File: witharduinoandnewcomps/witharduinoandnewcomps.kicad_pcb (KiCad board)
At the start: 2 copper layers, 60 x 90 mm, 20 parts, among them J1 FH34SRJ-24S-0.5SH_99_, Q2 ZXM61N03F, Q3 ZXM61N03F, SW1 Button-THT - 2-1825910-7

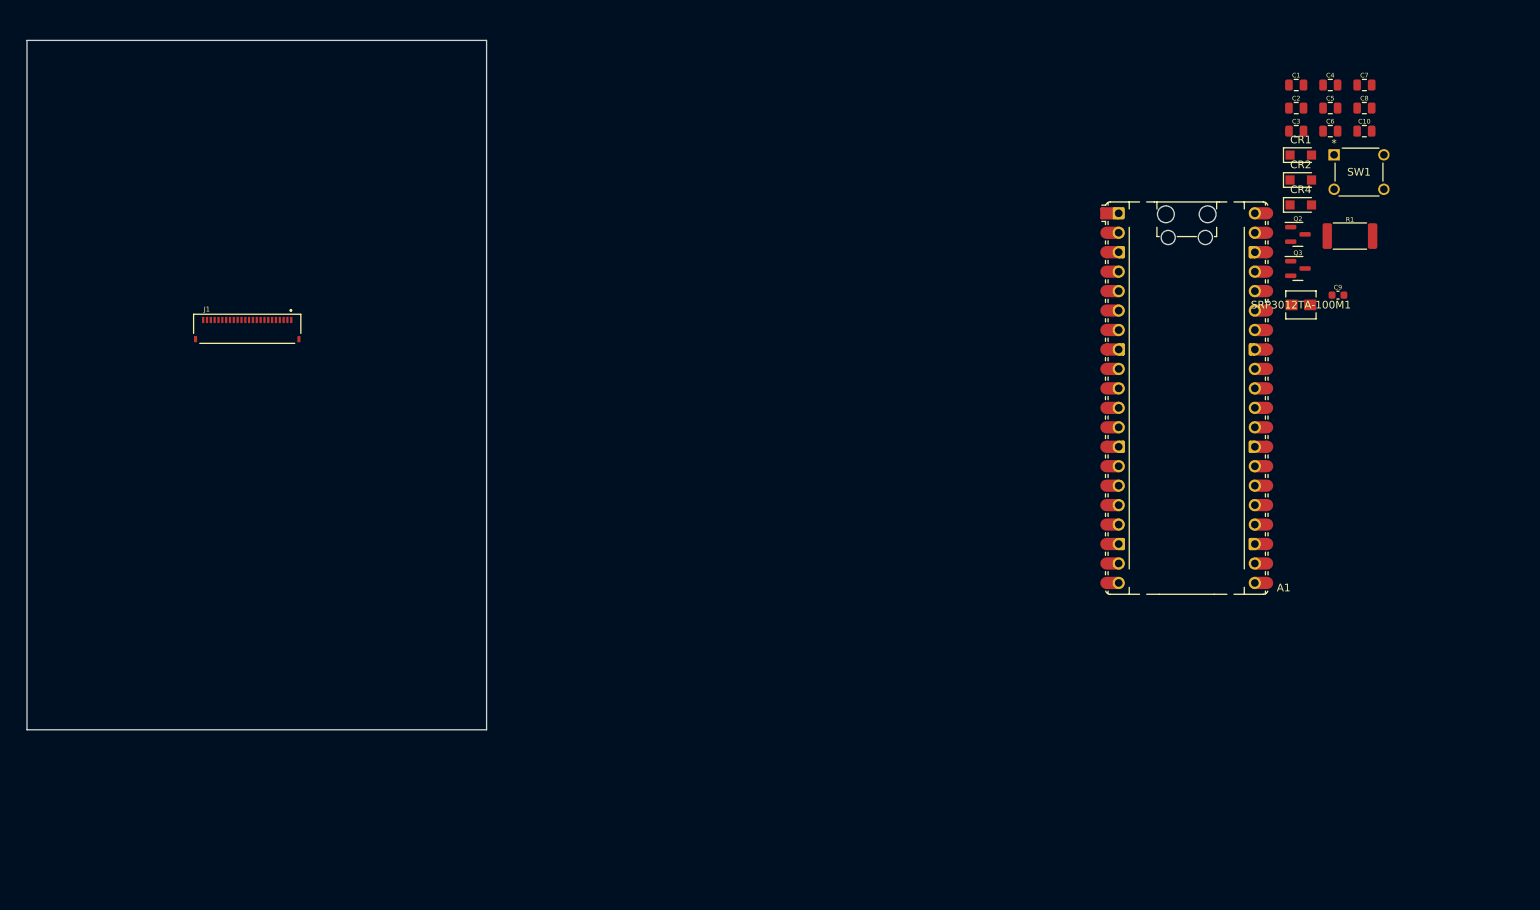
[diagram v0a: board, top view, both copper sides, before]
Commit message: Nov22
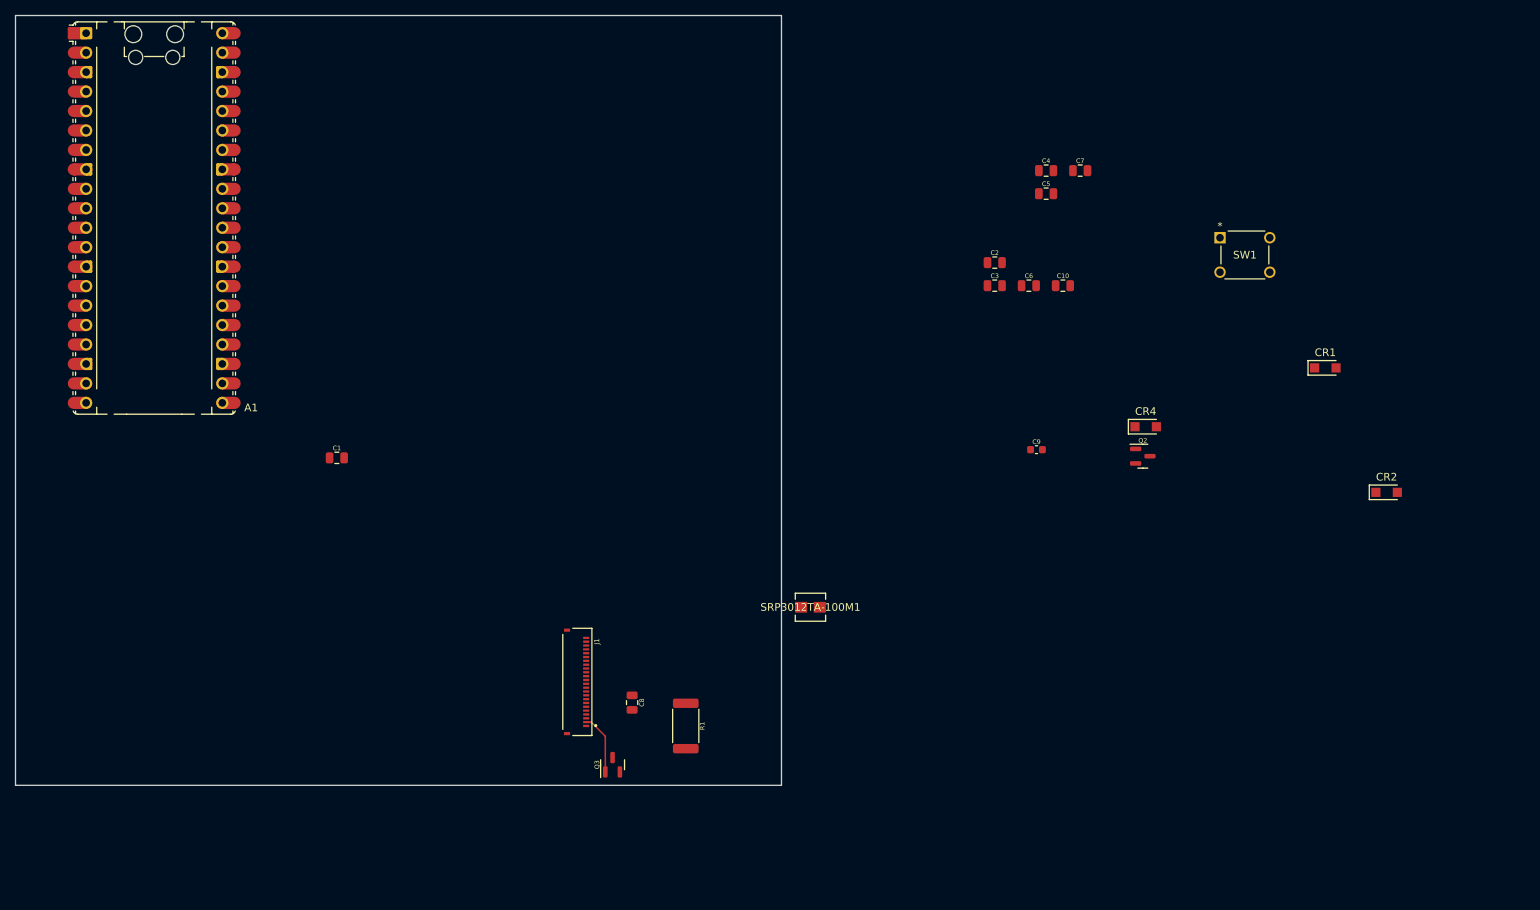
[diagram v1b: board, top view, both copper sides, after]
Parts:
- moved A1 136.8 mm to (44.6, 53.2)
- moved C1 134.4 mm to (68.5, 84.5)
- moved C8 123.1 mm to (107.0, 116.5), turned to -90 degrees
- moved Q3 110.5 mm to (104.5, 124.6), turned to 90 degrees
- moved R1 107.7 mm to (114.0, 119.5), turned to -90 degrees
- moved SRP3012TA-100M1 75.2 mm to (130.3, 104.0)
- moved J1 63.1 mm to (99.8, 113.8), turned to -90 degrees
- moved C6 44.2 mm to (158.8, 62.0)
- moved C9 44.2 mm to (159.8, 83.4)
- moved C10 44.2 mm to (163.2, 62.0)
- moved C2 44.2 mm to (154.3, 59.0)
- moved C3 44.2 mm to (154.3, 62.0)
- moved CR2 42.3 mm to (205.5, 89.0)
- moved C4 38.7 mm to (161.1, 47.0)
- moved C5 38.7 mm to (161.1, 50.0)
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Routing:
- net Net-(Q3-G): track 0.00 -> 7.92 mm
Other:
- board size 60 x 90 mm -> 100 x 100.5 mm

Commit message: laid out pcb
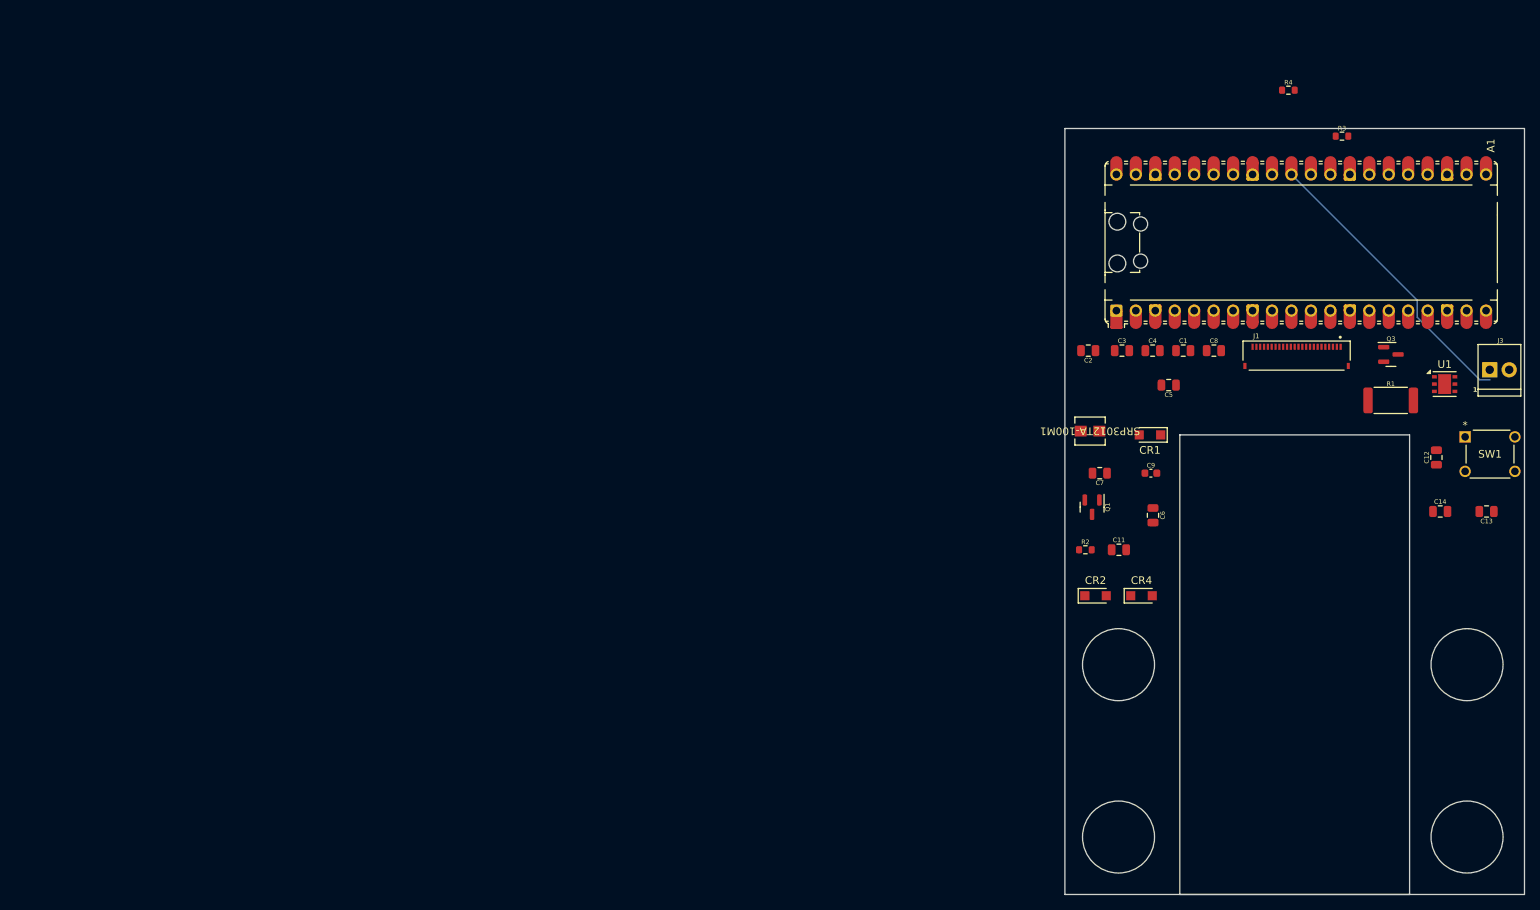
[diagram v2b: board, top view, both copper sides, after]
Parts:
- removed C10: 4u7, rsx_capacitors:C_0805_2012Metric
- removed Q2: ZXM61N03F, rsx_packages_TO_SOT:SOT-23
- added C11: 10u, rsx_capacitors:C_0805_2012Metric, F.Cu at (170.6, 96.5)
- added C12: 1u, rsx_capacitors:C_0805_2012Metric, F.Cu at (212.0, 84.5)
- added C13: 1u, rsx_capacitors:C_0805_2012Metric, F.Cu at (218.6, 91.5)
- added C14: 4u7, rsx_capacitors:C_0805_2012Metric, F.Cu at (212.5, 91.5)
- added J3: Screw_Terminal_2x2.54, rsx_headers_screw:Wurth_691210910002, F.Cu at (219.7, 73.0)
- added Q1: ZXM61N03F, rsx_packages_TO_SOT:SOT-23, F.Cu at (167.1, 90.9)
- added R2: 10k, rsx_resistors:R_0603_1608Metric, F.Cu at (166.2, 96.5)
- added R3: 249K_0.1%, rsx_resistors:R_0603_1608Metric, F.Cu at (199.7, 42.5)
- added R4: 1M, rsx_resistors:R_0603_1608Metric, F.Cu at (192.7, 36.5)
- added U1: LDO40LPU33RY, Package_DFN_QFN:DFN-6-1EP_3x3mm_P0.95mm_EP1.7x2.6mm, F.Cu at (213.1, 74.9)
- moved A1 149.8 mm to (194.3, 56.4), turned to 90 degrees
- moved Q3 114.9 mm to (206.1, 71.0), turned to 0 degrees
- moved C1 111.4 mm to (178.9, 70.5)
- moved J1 103.1 mm to (193.8, 71.2), turned to 0 degrees
- moved R1 101.4 mm to (206.0, 77.0), turned to 0 degrees
- moved C8 88.8 mm to (182.9, 70.5), turned to 0 degrees
- moved SRP3012TA-100M1 43.1 mm to (166.8, 81.0), turned to 180 degrees
- moved SW1 41.2 mm to (222.2, 86.3)
- moved CR2 40.3 mm to (167.5, 102.5)
- moved C7 39.6 mm to (168.1, 86.5), turned to 180 degrees
- moved C6 34.1 mm to (175.0, 92.0), turned to -90 degrees
- moved C5 29.7 mm to (177.1, 75.0), turned to 180 degrees
- moved C4 27.3 mm to (174.9, 70.5)
- moved CR1 24.5 mm to (174.6, 81.5), turned to 180 degrees
- moved CR4 22.1 mm to (173.5, 102.5)
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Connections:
- A1 pad 13: GNDPWR -> GND
- A1 pad 18: GNDPWR -> GND
- A1 pad 23: GNDPWR -> GND
- A1 pad 28: GNDPWR -> GND
- A1 pad 3: GNDPWR -> GND
- A1 pad 36: power -> unconnected-(A1-3V3-Pad36)_1
- A1 pad 38: GNDPWR -> GND
- A1 pad 39: Net-(A1-VSYS) -> 3.3v in power
- A1 pad 8: GNDPWR -> GND
- C1 pad 1: GNDPWR -> GND
- C2 pad 1: GNDPWR -> GND
- C2 pad 2: unconnected-(C2-Pad2) -> Net-(C2-Pad2)
- C3 pad 1: GNDPWR -> GND
- C4 pad 1: GNDPWR -> GND
- C5 pad 1: GNDPWR -> GND
- C6 pad 1: GNDPWR -> GND
- C6 pad 2: unconnected-(C2-Pad2) -> Net-(C6-Pad2)
- C7 pad 1: GNDPWR -> GND
- C8 pad 1: GNDPWR -> GND
- C9 pad 2: GNDPWR -> GND
- CR2 pad 1: GNDPWR -> GND
- CR4 pad 2: unconnected-(C2-Pad2) -> Net-(C6-Pad2)
- J1 pad 17: GNDPWR -> GND
- J1 pad 23: unconnected-(C2-Pad2) -> Net-(C6-Pad2)
- J1 pad 24: unconnected-(C2-Pad2) -> Net-(C2-Pad2)
- J1 pad S1: unconnected-(C2-Pad2) -> GND
- J1 pad S2: unconnected-(C2-Pad2) -> GND
- R1 pad 1: GNDPWR -> GND
- SW1 pad 1: power -> +12V
- SW1 pad 2: Net-(A1-VSYS) -> Net-(U1-EN)
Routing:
- net Net-(A1-GPIO26_ADC0): track 0.00 -> 38.3 mm
- net Net-(Q3-G): track 7.92 -> 0.00 mm
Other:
- board size 100 x 100.5 mm -> 60 x 100 mm
